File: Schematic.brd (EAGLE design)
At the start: 84 x 96 mm, 64 parts

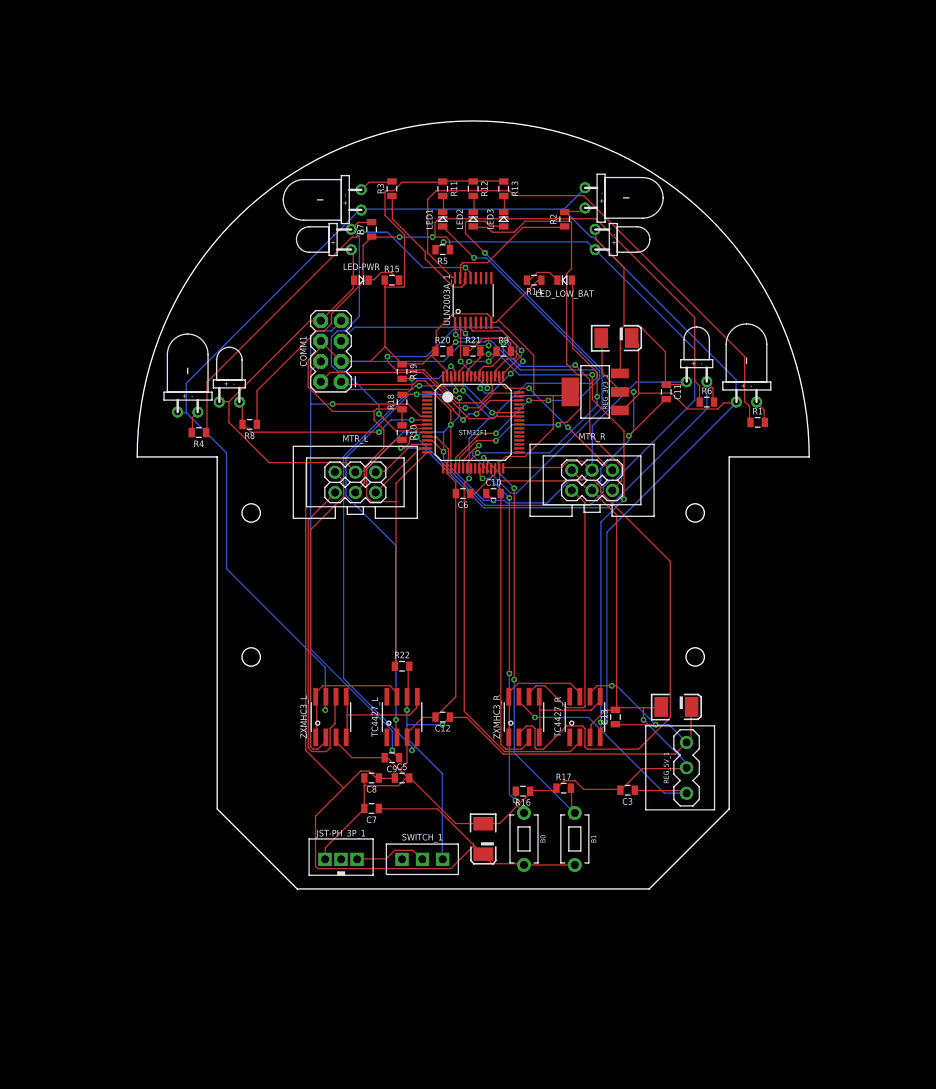
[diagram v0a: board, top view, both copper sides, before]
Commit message: 013120meeting
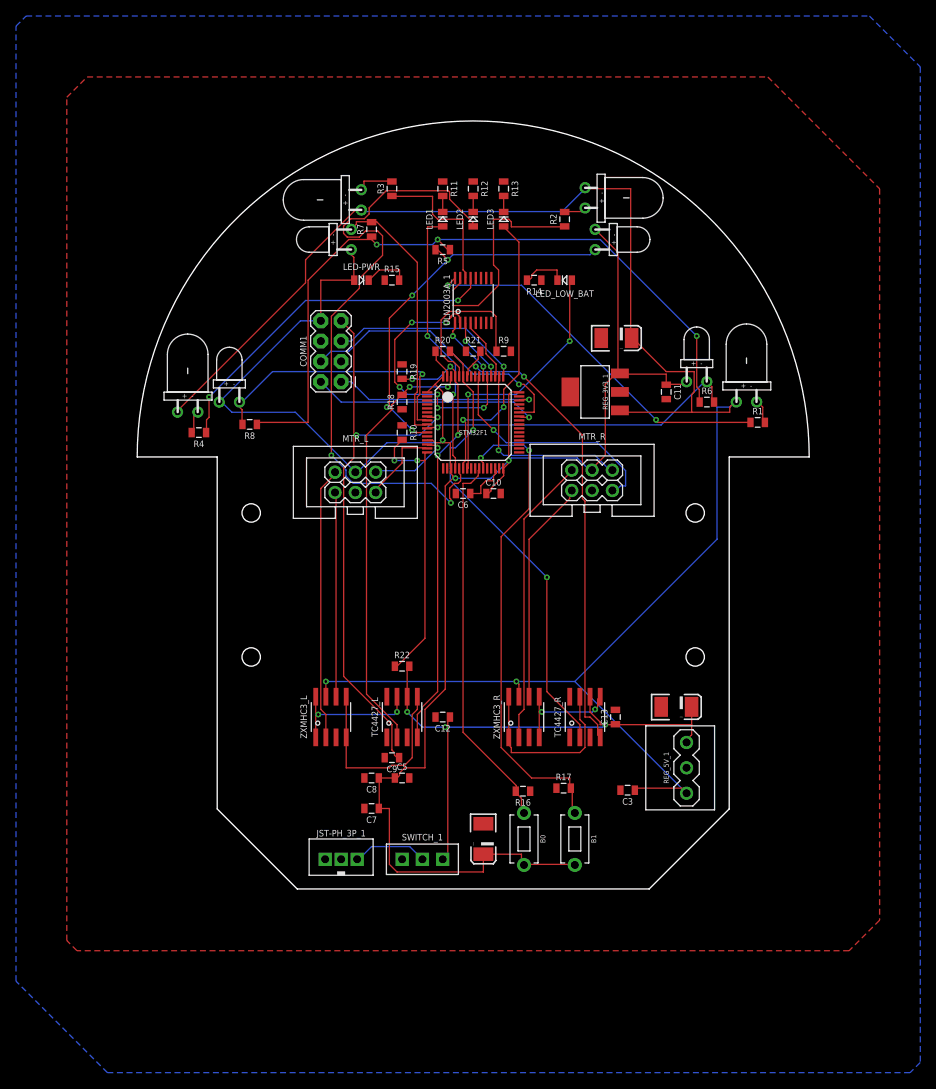
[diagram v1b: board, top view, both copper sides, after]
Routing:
- net GND: track 425.7 -> 4.02 mm, vias 4 -> 0
- net +3V3: track 295.1 -> 242.1 mm, vias 5 -> 3
- net RPWM_A: track 99.3 -> 57.8 mm, vias 3 -> 2
- net RE_LF: track 90.4 -> 49.1 mm, vias 2 -> 4
- net RMTR+: track 64.7 -> 36.2 mm
- net LED3: track 63.3 -> 36.2 mm
- net LED2: track 56.7 -> 80.9 mm
- net +5V: track 249.3 -> 225.9 mm
- net EM_RD: track 31.0 -> 8.01 mm
- net EM_LD: track 11.1 -> 33.4 mm, vias 2 -> 6
- net N$1: track 68.7 -> 46.5 mm, vias 0 -> 2
- net V+: track 89.9 -> 70.5 mm, vias 4 -> 3
- net LMTR-: track 43.2 -> 25.6 mm
- net LED1: track 51.5 -> 34.1 mm, vias 4 -> 2
- net RE_LD: track 57.6 -> 40.5 mm
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- added copper zone on layer 1, net GND
- added copper zone on layer 16, net GND
